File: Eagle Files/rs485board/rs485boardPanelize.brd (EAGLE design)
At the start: 63.5 x 76.7 mm, 100 parts, among them IC1 XC6206P332MR, IC2 MP2562, J1 AVR_SPI_PROG_3X2PTH, J2 RA 6Pin SMD, Q1 CJ3404, Q2 CJ3404, Q3 CJ3404, U1 ATMEGA328P_TQFP, U2 LIS3DH, U3 SP485, X1 RJ45-8P8C-8L-B, X3 RJ45-8P8C-8L-B, Y1 16MHz

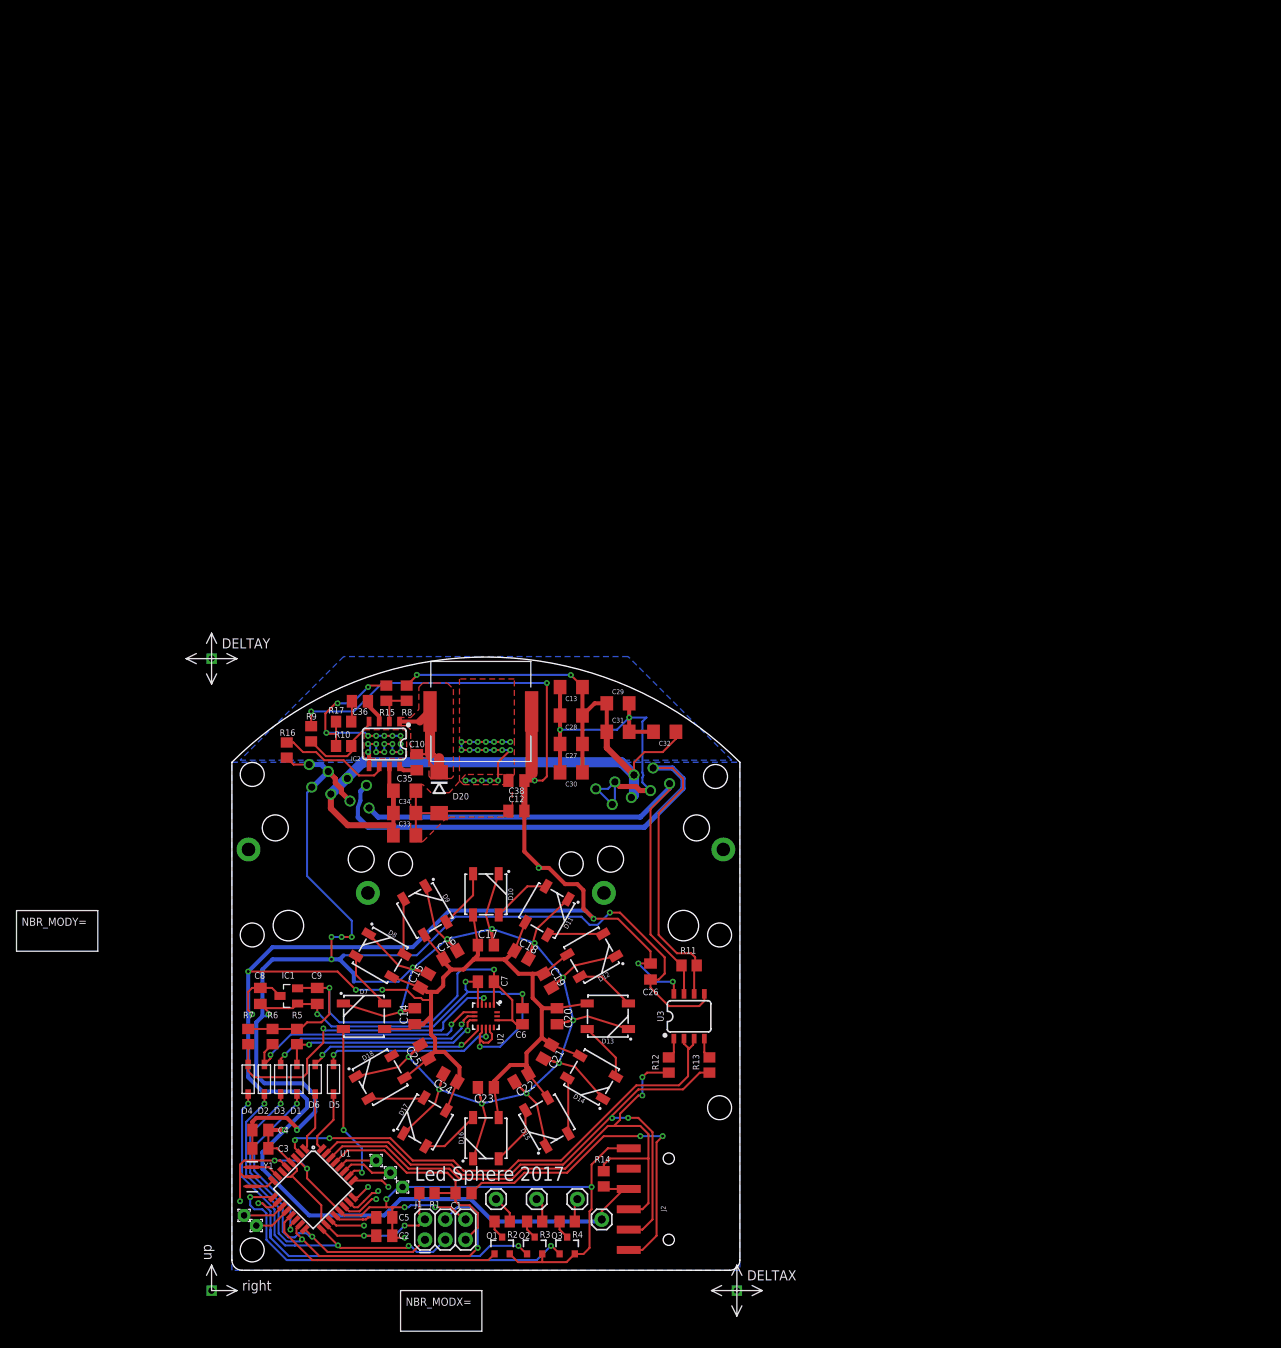
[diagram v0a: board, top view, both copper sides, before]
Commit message: clean up 2*2
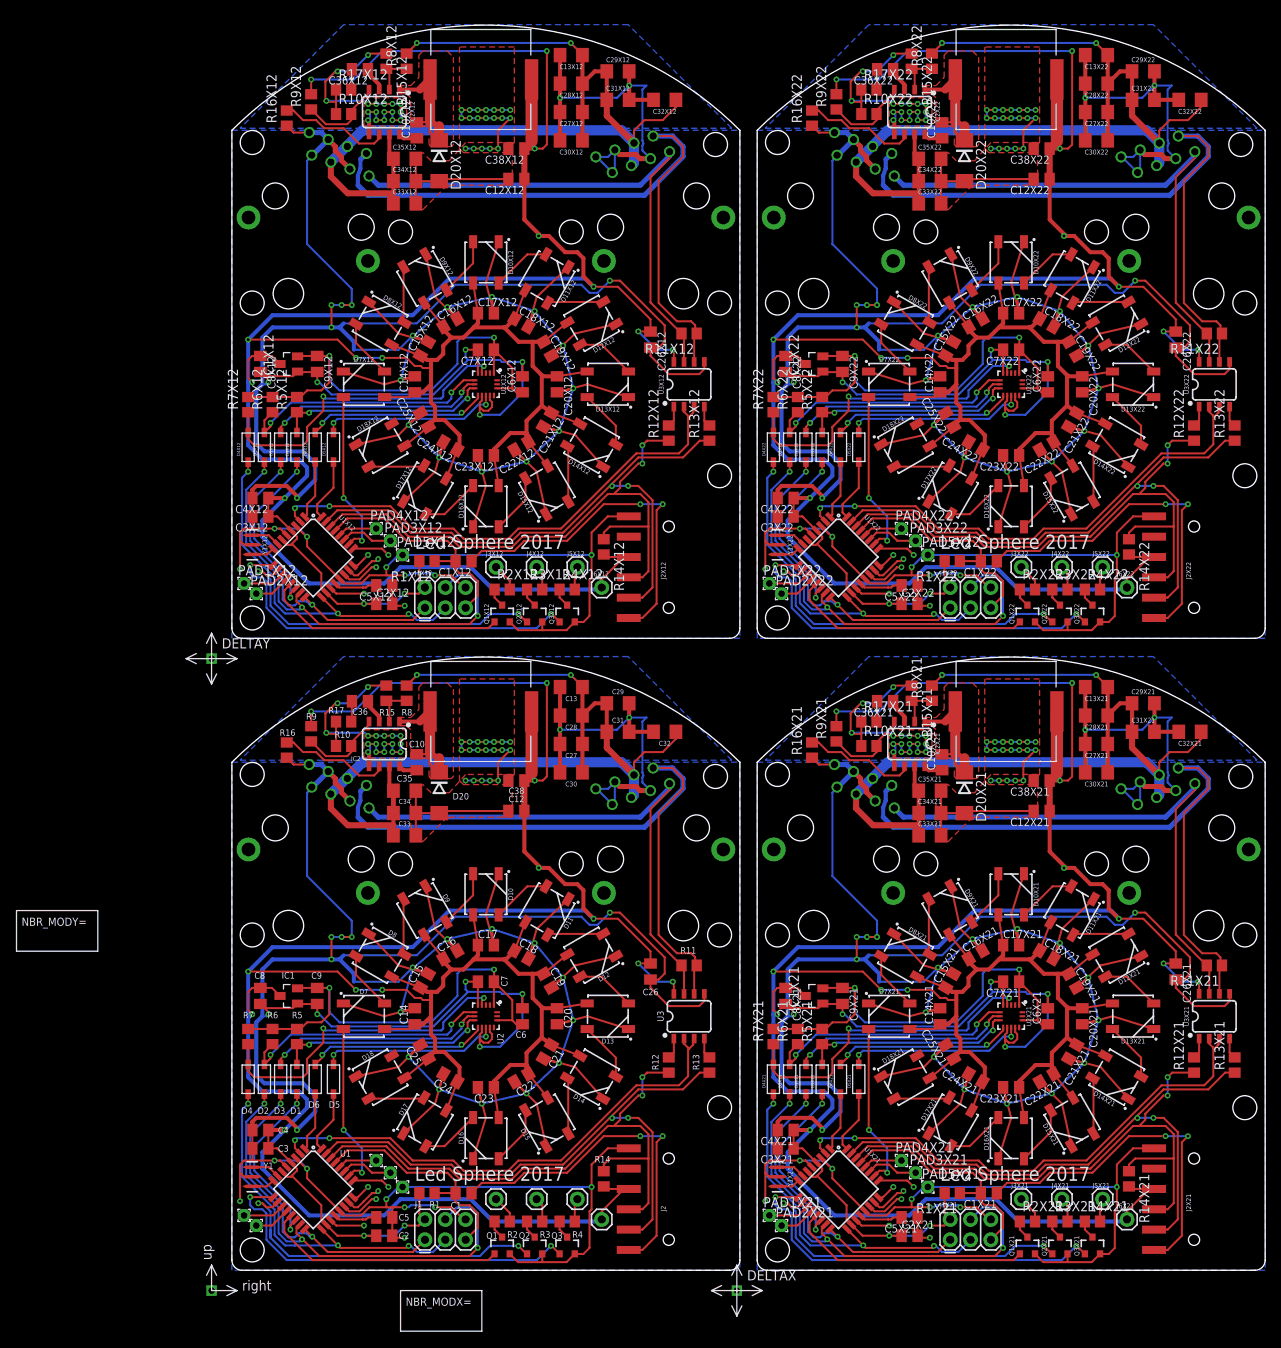
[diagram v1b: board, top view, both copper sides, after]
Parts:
- added C10X12, C10X21, C10X22, C14X12, C14X21, C14X22, C15X12, C15X21, C15X22, C16X12, C16X21, C16X22, C17X12, C17X21, C17X22, C18X12, C18X21, C18X22, C19X12, C19X21, C19X22, C1X12, C1X21, C1X22, C20X12, C20X21, C20X22, C21X12, C21X21, C21X22, C22X12, C22X21, C22X22, C23X12, C23X21, C23X22, C24X12, C24X21, C24X22, C25X12, C25X21, C25X22, C26X12, C26X21, C26X22, C3X12, C3X21, C3X22, C4X12, C4X21, C4X22, C5X12, C5X21, C5X22, C7X12, C7X21, C7X22, C8X12, C8X21, C8X22, C9X12, C9X21, C9X22: 0.1uF, resistor:C0805K
- added C12X12, C12X21, C12X22, C2X12, C2X21, C2X22, C38X12, C38X21, C38X22, C6X12, C6X21, C6X22: 10uF, resistor:C0805K
- added C13X12, C13X21, C13X22, C27X12, C27X21, C27X22, C28X12, C28X21, C28X22, C29X12, C29X21, C29X22, C30X12, C30X21, C30X22, C31X12, C31X21, C31X22, C32X12, C32X21, C32X22, C33X12, C33X21, C33X22, C34X12, C34X21, C34X22, C35X12, C35X21, C35X22: 1uF 100V, SparkFun-Capacitors:1206
- added C36X12, C36X21, C36X22: 150pF, resistor:C0805K
- added D10X12, D10X21, D10X22, D11X12, D11X21, D11X22, D12X12, D12X21, D12X22, D13X12, D13X21, D13X22, D14X12, D14X21, D14X22, D15X12, D15X21, D15X22, D16X12, D16X21, D16X22, D17X12, D17X21, D17X22, D18X12, D18X21, D18X22, D7X12, D7X21, D7X22, D8X12, D8X21, D8X22, D9X12, D9X21, D9X22: WS2812B, SparkFun-LED:WS2812B
- added D1X12, D1X21, D1X22, D2X12, D2X21, D2X22, D3X12, D3X21, D3X22, D4X12, D4X21, D4X22, D5X12, D5X21, D5X22, D6X12, D6X21, D6X22: 5819, adafruit:SOD-123
- added D20X12, D20X21, D20X22: B280-13-F, diode:DO214AA
- added IC1X12, IC1X21, IC1X22: XC6206P332MR, linear:SOT23
- added IC2X12, IC2X21, IC2X22: MP2562, misc:SO08
- added J1X12, J1X21, J1X22: AVR_SPI_PROG_3X2PTH, SparkFun-Connectors:2X3
- added J2X12, J2X21, J2X22: RA 6Pin SMD, SparkFun-Connectors:1X06-SMD_RA_MALE
- added J3X12, J3X21, J3X22, J4X12, J4X21, J4X22, J5X12, J5X21, J5X22, J6X12, J6X21, J6X22: (no value), SparkFun-Connectors:1X01
- added L1X12, L1X21, L1X22: 15uH, misc:SLF12575
- added PAD1X12, PAD1X21, PAD1X22, PAD2X12, PAD2X21, PAD2X22, PAD3X12, PAD3X21, PAD3X22, PAD4X12, PAD4X21, PAD4X22, PAD5X12, PAD5X21, PAD5X22: (no value), wirepad:1,6/0,8
- added Q1X12, Q1X21, Q1X22, Q2X12, Q2X21, Q2X22, Q3X12, Q3X21, Q3X22: CJ3404, SparkFun-DiscreteSemi:SOT23-3
- added R10X12, R10X21, R10X22: 40.2k, resistor:R0805
- added R11X12, R11X21, R11X22: 120, resistor:R0805
- added R12X12, R12X21, R12X22, R13X12, R13X21, R13X22: 1K, resistor:R0805
- added R14X12, R14X21, R14X22, R1X12, R1X21, R1X22, R5X12, R5X21, R5X22, R6X12, R6X21, R6X22, R7X12, R7X21, R7X22: 10K, resistor:R0805
- added R15X12, R15X21, R15X22: 17.4K, resistor:R0805
- added R16X12, R16X21, R16X22: 200K, resistor:R0805
- added R17X12, R17X21, R17X22: 158K, resistor:R0805
- added R2X12, R2X21, R2X22, R3X12, R3X21, R3X22, R4X12, R4X21, R4X22: DNP, resistor:R0805
- added R8X12, R8X21, R8X22: 100K, resistor:R0805
- added R9X12, R9X21, R9X22: 210K, resistor:R0805
- added U1X12, U1X21, U1X22: ATMEGA328P_TQFP, SparkFun-IC-Microcontroller:TQFP32-08
- added U2X12, U2X21, U2X22: LIS3DH, SparkFun-Sensors:LGA-16-3X3
- added U3X12, U3X21, U3X22: SP485, SparkFun-IC-Comms:SO08
- added X1X12, X1X21, X1X22, X3X12, X3X21, X3X22: RJ45-8P8C-8L-B, myownParts:RJ45-SHIELD-DS1128-S80BP
- added Y1X12, Y1X21, Y1X22: 16MHz, SparkFun-Clocks:RESONATOR-SMD-3.2X1.3
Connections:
- new net +24VX12: C13X12.1, C27X12.1, C28X12.1, C29X12.1, C30X12.1, C31X12.1, C32X12.1, C33X12.1, C34X12.1, C35X12.1, IC2X12.7, R8X12.2, X1X12.4, X1X12.5, X3X12.4, X3X12.5
- new net +24VX21: C13X21.1, C27X21.1, C28X21.1, C29X21.1, C30X21.1, C31X21.1, C32X21.1, C33X21.1, C34X21.1, C35X21.1, IC2X21.7, R8X21.2, X1X21.4, X1X21.5, X3X21.4, X3X21.5
- new net +24VX22: C13X22.1, C27X22.1, C28X22.1, C29X22.1, C30X22.1, C31X22.1, C32X22.1, C33X22.1, C34X22.1, C35X22.1, IC2X22.7, R8X22.2, X1X22.4, X1X22.5, X3X22.4, X3X22.5
- new net +3V3X12: C6X12.1, C7X12.1, C9X12.1, IC1X12.2, R5X12.2, R6X12.2, R7X12.2, U2X12.1, U2X12.14
- new net +3V3X21: C6X21.1, C7X21.1, C9X21.1, IC1X21.2, R5X21.2, R6X21.2, R7X21.2, U2X21.1, U2X21.14
- new net +3V3X22: C6X22.1, C7X22.1, C9X22.1, IC1X22.2, R5X22.2, R6X22.2, R7X22.2, U2X22.1, U2X22.14
- new net +5VX12: C12X12.1, C14X12.1, C15X12.1, C16X12.1, C17X12.1, C18X12.1, C19X12.1, C20X12.1, C21X12.1, C22X12.1, C23X12.1, C24X12.1, C25X12.1, C26X12.1, C2X12.1, C38X12.1, C3X12.1, C4X12.1, C8X12.1, D10X12.1, D11X12.1, D12X12.1, D13X12.1, D14X12.1, D15X12.1, D16X12.1, D17X12.1, D18X12.1, D7X12.1, D8X12.1, D9X12.1, IC1X12.3, J1X12.2, J2X12.4, J6X12.1, L1X12.P$2, R14X12.2, R1X12.2, R9X12.2, U1X12.18, U1X12.4, U1X12.6, U3X12.8
- new net +5VX21: C12X21.1, C14X21.1, C15X21.1, C16X21.1, C17X21.1, C18X21.1, C19X21.1, C20X21.1, C21X21.1, C22X21.1, C23X21.1, C24X21.1, C25X21.1, C26X21.1, C2X21.1, C38X21.1, C3X21.1, C4X21.1, C8X21.1, D10X21.1, D11X21.1, D12X21.1, D13X21.1, D14X21.1, D15X21.1, D16X21.1, D17X21.1, D18X21.1, D7X21.1, D8X21.1, D9X21.1, IC1X21.3, J1X21.2, J2X21.4, J6X21.1, L1X21.P$2, R14X21.2, R1X21.2, R9X21.2, U1X21.18, U1X21.4, U1X21.6, U3X21.8
- new net +5VX22: C12X22.1, C14X22.1, C15X22.1, C16X22.1, C17X22.1, C18X22.1, C19X22.1, C20X22.1, C21X22.1, C22X22.1, C23X22.1, C24X22.1, C25X22.1, C26X22.1, C2X22.1, C38X22.1, C3X22.1, C4X22.1, C8X22.1, D10X22.1, D11X22.1, D12X22.1, D13X22.1, D14X22.1, D15X22.1, D16X22.1, D17X22.1, D18X22.1, D7X22.1, D8X22.1, D9X22.1, IC1X22.3, J1X22.2, J2X22.4, J6X22.1, L1X22.P$2, R14X22.2, R1X22.2, R9X22.2, U1X22.18, U1X22.4, U1X22.6, U3X22.8
- new net A3X12: D7X12.4, U1X12.26
- new net A3X21: D7X21.4, U1X21.26
- new net A3X22: D7X22.4, U1X22.26
- new net A4X12: PAD3X12.1, U1X12.27
- new net A4X21: PAD3X21.1, U1X21.27
- new net A4X22: PAD3X22.1, U1X22.27
- new net A5X12: PAD4X12.1, U1X12.28
- new net A5X21: PAD4X21.1, U1X21.28
- new net A5X22: PAD4X22.1, U1X22.28
- new net AREFX12: C5X12.2, U1X12.20
- new net AREFX21: C5X21.2, U1X21.20
- new net AREFX22: C5X22.2, U1X22.20
- new net BSTX12: C10X12.1, IC2X12.8
- new net BSTX21: C10X21.1, IC2X21.8
- new net BSTX22: C10X22.1, IC2X22.8
- new net COMPX12: C36X12.1, IC2X12.3
- new net COMPX21: C36X21.1, IC2X21.3
- new net COMPX22: C36X22.1, IC2X22.3
- new net D2X12: D5X12.C, U1X12.32
- new net D2X21: D5X21.C, U1X21.32
- new net D2X22: D5X22.C, U1X22.32
- new net D3X12: D6X12.C, U1X12.1
- new net D3X21: D6X21.C, U1X21.1
- new net D3X22: D6X22.C, U1X22.1
- new net D5X12: Q3X12.1, U1X12.9
- new net D5X21: Q3X21.1, U1X21.9
- new net D5X22: Q3X22.1, U1X22.9
- new net D6X12: Q2X12.1, U1X12.10
- new net D6X21: Q2X21.1, U1X21.10
- new net D6X22: Q2X22.1, U1X22.10
- new net D7X12: PAD1X12.1, U1X12.11
- new net D7X21: PAD1X21.1, U1X21.11
- new net D7X22: PAD1X22.1, U1X22.11
- new net D8X12: PAD2X12.1, U1X12.12
- new net D8X21: PAD2X21.1, U1X21.12
- new net D8X22: PAD2X22.1, U1X22.12
- new net D9X12: Q1X12.1, U1X12.13
- new net D9X21: Q1X21.1, U1X21.13
- new net D9X22: Q1X22.1, U1X22.13
- new net DIRX12: U1X12.2, U3X12.2, U3X12.3
- new net DIRX21: U1X21.2, U3X21.2, U3X21.3
- new net DIRX22: U1X22.2, U3X22.2, U3X22.3
- new net ENX12: IC2X12.2, R15X12.2, R8X12.1
- new net ENX21: IC2X21.2, R15X21.2, R8X21.1
- new net ENX22: IC2X22.2, R15X22.2, R8X22.1
- new net FBX12: IC2X12.4, R10X12.2, R9X12.1
- new net FBX21: IC2X21.4, R10X21.2, R9X21.1
- new net FBX22: IC2X22.4, R10X22.2, R9X22.1
- new net FREQX12: IC2X12.6, R16X12.2
- new net FREQX21: IC2X21.6, R16X21.2
- new net FREQX22: IC2X22.6, R16X22.2
- new net GNDX12: C12X12.2, C13X12.2, C14X12.2, C15X12.2, C16X12.2, C17X12.2, C18X12.2, C19X12.2, C20X12.2, C21X12.2, C22X12.2, C23X12.2, C24X12.2, C25X12.2, C26X12.2, C27X12.2, C28X12.2, C29X12.2, C2X12.2, C30X12.2, C31X12.2, C32X12.2, C33X12.2, C34X12.2, C35X12.2, C38X12.2, C3X12.2, C4X12.2, C5X12.1, C6X12.2, C7X12.2, C8X12.2, C9X12.2, D10X12.3, D11X12.3, D12X12.3, D13X12.3, D14X12.3, D15X12.3, D16X12.3, D17X12.3, D18X12.3, D20X12.A, D7X12.3, D8X12.3, D9X12.3, IC1X12.1, IC2X12.5, J1X12.6, J2X12.6, PAD5X12.1, Q1X12.2, Q2X12.2, Q3X12.2, R10X12.1, R15X12.1, R16X12.1, R17X12.1, U1X12.21, U1X12.3, U1X12.5, U2X12.10, U2X12.12, U2X12.5, U3X12.5, X1X12.3, X1X12.6, X1X12.7, X1X12.8, X3X12.3, X3X12.6, X3X12.7, X3X12.8, Y1X12.2
- new net GNDX21: C12X21.2, C13X21.2, C14X21.2, C15X21.2, C16X21.2, C17X21.2, C18X21.2, C19X21.2, C20X21.2, C21X21.2, C22X21.2, C23X21.2, C24X21.2, C25X21.2, C26X21.2, C27X21.2, C28X21.2, C29X21.2, C2X21.2, C30X21.2, C31X21.2, C32X21.2, C33X21.2, C34X21.2, C35X21.2, C38X21.2, C3X21.2, C4X21.2, C5X21.1, C6X21.2, C7X21.2, C8X21.2, C9X21.2, D10X21.3, D11X21.3, D12X21.3, D13X21.3, D14X21.3, D15X21.3, D16X21.3, D17X21.3, D18X21.3, D20X21.A, D7X21.3, D8X21.3, D9X21.3, IC1X21.1, IC2X21.5, J1X21.6, J2X21.6, PAD5X21.1, Q1X21.2, Q2X21.2, Q3X21.2, R10X21.1, R15X21.1, R16X21.1, R17X21.1, U1X21.21, U1X21.3, U1X21.5, U2X21.10, U2X21.12, U2X21.5, U3X21.5, X1X21.3, X1X21.6, X1X21.7, X1X21.8, X3X21.3, X3X21.6, X3X21.7, X3X21.8, Y1X21.2
- new net GNDX22: C12X22.2, C13X22.2, C14X22.2, C15X22.2, C16X22.2, C17X22.2, C18X22.2, C19X22.2, C20X22.2, C21X22.2, C22X22.2, C23X22.2, C24X22.2, C25X22.2, C26X22.2, C27X22.2, C28X22.2, C29X22.2, C2X22.2, C30X22.2, C31X22.2, C32X22.2, C33X22.2, C34X22.2, C35X22.2, C38X22.2, C3X22.2, C4X22.2, C5X22.1, C6X22.2, C7X22.2, C8X22.2, C9X22.2, D10X22.3, D11X22.3, D12X22.3, D13X22.3, D14X22.3, D15X22.3, D16X22.3, D17X22.3, D18X22.3, D20X22.A, D7X22.3, D8X22.3, D9X22.3, IC1X22.1, IC2X22.5, J1X22.6, J2X22.6, PAD5X22.1, Q1X22.2, Q2X22.2, Q3X22.2, R10X22.1, R15X22.1, R16X22.1, R17X22.1, U1X22.21, U1X22.3, U1X22.5, U2X22.10, U2X22.12, U2X22.5, U3X22.5, X1X22.3, X1X22.6, X1X22.7, X1X22.8, X3X22.3, X3X22.6, X3X22.7, X3X22.8, Y1X22.2
- new net INT1X12: D5X12.A, U2X12.11
- new net INT1X21: D5X21.A, U2X21.11
- new net INT1X22: D5X22.A, U2X22.11
- new net INT2X12: D6X12.A, U2X12.9
- new net INT2X21: D6X21.A, U2X21.9
- new net INT2X22: D6X22.A, U2X22.9
- new net MISOX12: D3X12.C, J1X12.1, U1X12.16
- new net MISOX21: D3X21.C, J1X21.1, U1X21.16
- new net MISOX22: D3X22.C, J1X22.1, U1X22.16
- new net MISO_3.3VX12: D3X12.A, U2X12.7
- new net MISO_3.3VX21: D3X21.A, U2X21.7
- new net MISO_3.3VX22: D3X22.A, U2X22.7
- new net MOSIX12: D2X12.C, J1X12.4, U1X12.15
- new net MOSIX21: D2X21.C, J1X21.4, U1X21.15
- new net MOSIX22: D2X22.C, J1X22.4, U1X22.15
- new net MOSI_3.3VX12: D2X12.A, R6X12.1, U2X12.6
- new net MOSI_3.3VX21: D2X21.A, R6X21.1, U2X21.6
- new net MOSI_3.3VX22: D2X22.A, R6X22.1, U2X22.6
- new net N$10X12: D10X12.2, D11X12.4
- new net N$10X21: D10X21.2, D11X21.4
- new net N$10X22: D10X22.2, D11X22.4
- new net N$11X12: D11X12.2, D12X12.4
- new net N$11X21: D11X21.2, D12X21.4
- new net N$11X22: D11X22.2, D12X22.4
- new net N$12X12: D12X12.2, D13X12.4
- new net N$12X21: D12X21.2, D13X21.4
- new net N$12X22: D12X22.2, D13X22.4
- new net N$13X12: D13X12.2, D14X12.4
- new net N$13X21: D13X21.2, D14X21.4
- new net N$13X22: D13X22.2, D14X22.4
- new net N$14X12: D14X12.2, D15X12.4
- new net N$14X21: D14X21.2, D15X21.4
- new net N$14X22: D14X22.2, D15X22.4
- new net N$15X12: D15X12.2, D16X12.4
- new net N$15X21: D15X21.2, D16X21.4
- new net N$15X22: D15X22.2, D16X22.4
- new net N$16X12: D16X12.2, D17X12.4
- new net N$16X21: D16X21.2, D17X21.4
- new net N$16X22: D16X22.2, D17X22.4
- new net N$17X12: D17X12.2, D18X12.4
- new net N$17X21: D17X21.2, D18X21.4
- new net N$17X22: D17X22.2, D18X22.4
- new net N$1X12: Q1X12.3, R2X12.1
- new net N$1X21: Q1X21.3, R2X21.1
- new net N$1X22: Q1X22.3, R2X22.1
- new net N$25X12: C36X12.2, R17X12.2
- new net N$25X21: C36X21.2, R17X21.2
- new net N$25X22: C36X22.2, R17X22.2
- new net N$2X12: D7X12.2, D8X12.4
- new net N$2X21: D7X21.2, D8X21.4
- new net N$2X22: D7X22.2, D8X22.4
- new net N$30X12: R12X12.2, U3X12.1
- new net N$30X21: R12X21.2, U3X21.1
- new net N$30X22: R12X22.2, U3X22.1
- new net N$31X12: R13X12.2, U3X12.4
- new net N$31X21: R13X21.2, U3X21.4
- new net N$31X22: R13X22.2, U3X22.4
- new net N$3X12: D8X12.2, D9X12.4
- new net N$3X21: D8X21.2, D9X21.4
- new net N$3X22: D8X22.2, D9X22.4
- new net N$4X12: J3X12.1, R2X12.2
- new net N$4X21: J3X21.1, R2X21.2
- new net N$4X22: J3X22.1, R2X22.2
- new net N$5X12: Q2X12.3, R3X12.1
- new net N$5X21: Q2X21.3, R3X21.1
- new net N$5X22: Q2X22.3, R3X22.1
- new net N$6X12: J4X12.1, R3X12.2
- new net N$6X21: J4X21.1, R3X21.2
- new net N$6X22: J4X22.1, R3X22.2
- new net N$7X12: Q3X12.3, R4X12.1
- new net N$7X21: Q3X21.3, R4X21.1
- new net N$7X22: Q3X22.3, R4X22.1
- new net N$8X12: J5X12.1, R4X12.2
- new net N$8X21: J5X21.1, R4X21.2
- new net N$8X22: J5X22.1, R4X22.2
- new net N$9X12: D10X12.4, D9X12.2
- new net N$9X21: D10X21.4, D9X21.2
- new net N$9X22: D10X22.4, D9X22.2
- new net RESETX12: C1X12.2, J1X12.5, R1X12.1, U1X12.29
- new net RESETX21: C1X21.2, J1X21.5, R1X21.1, U1X21.29
- new net RESETX22: C1X22.2, J1X22.5, R1X22.1, U1X22.29
- new net RESET_EXTX12: C1X12.1, J2X12.1
- new net RESET_EXTX21: C1X21.1, J2X21.1
- new net RESET_EXTX22: C1X22.1, J2X22.1
- new net RS485AX12: R11X12.1, U3X12.6, X1X12.2, X3X12.2
- new net RS485AX21: R11X21.1, U3X21.6, X1X21.2, X3X21.2
- new net RS485AX22: R11X22.1, U3X22.6, X1X22.2, X3X22.2
- new net RS485BX12: R11X12.2, U3X12.7, X1X12.1, X3X12.1
- new net RS485BX21: R11X21.2, U3X21.7, X1X21.1, X3X21.1
- new net RS485BX22: R11X22.2, U3X22.7, X1X22.1, X3X22.1
- new net RXX12: J2X12.3, R12X12.1, R14X12.1, U1X12.30
- new net RXX21: J2X21.3, R12X21.1, R14X21.1, U1X21.30
- new net RXX22: J2X22.3, R12X22.1, R14X22.1, U1X22.30
- new net SCKX12: D4X12.C, J1X12.3, U1X12.17
- new net SCKX21: D4X21.C, J1X21.3, U1X21.17
- new net SCKX22: D4X22.C, J1X22.3, U1X22.17
- new net SCK_3.3VX12: D4X12.A, R7X12.1, U2X12.4
- new net SCK_3.3VX21: D4X21.A, R7X21.1, U2X21.4
- new net SCK_3.3VX22: D4X22.A, R7X22.1, U2X22.4
- new net SSX12: D1X12.C, U1X12.14
- new net SSX21: D1X21.C, U1X21.14
- new net SSX22: D1X22.C, U1X22.14
- new net SS_3.3VX12: D1X12.A, R5X12.1, U2X12.8
- new net SS_3.3VX21: D1X21.A, R5X21.1, U2X21.8
- new net SS_3.3VX22: D1X22.A, R5X22.1, U2X22.8
- new net SWX12: C10X12.2, D20X12.C, IC2X12.1, L1X12.P$1
- new net SWX21: C10X21.2, D20X21.C, IC2X21.1, L1X21.P$1
- new net SWX22: C10X22.2, D20X22.C, IC2X22.1, L1X22.P$1
- new net TXX12: J2X12.2, R13X12.1, U1X12.31
- new net TXX21: J2X21.2, R13X21.1, U1X21.31
- new net TXX22: J2X22.2, R13X22.1, U1X22.31
- new net XTAL1X12: U1X12.7, Y1X12.1
- new net XTAL1X21: U1X21.7, Y1X21.1
- new net XTAL1X22: U1X22.7, Y1X22.1
- new net XTAL2X12: U1X12.8, Y1X12.3
- new net XTAL2X21: U1X21.8, Y1X21.3
- new net XTAL2X22: U1X22.8, Y1X22.3
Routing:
- net GNDX22: track 0.00 -> 654.9 mm, vias 0 -> 70
- net GNDX21: track 0.00 -> 654.9 mm, vias 0 -> 70
- net GNDX12: track 0.00 -> 654.9 mm, vias 0 -> 70
- net +5VX21: track 0.00 -> 417.0 mm, vias 0 -> 14
- net +5VX22: track 0.00 -> 417.0 mm, vias 0 -> 14
- net +5VX12: track 0.00 -> 417.0 mm, vias 0 -> 14
- net +24VX22: track 0.00 -> 119.4 mm, vias 0 -> 2
- net +24VX12: track 0.00 -> 119.4 mm, vias 0 -> 2
- net +24VX21: track 0.00 -> 119.4 mm, vias 0 -> 2
- net RS485AX21: track 0.00 -> 88.7 mm
- net RS485AX22: track 0.00 -> 88.7 mm
- net RS485AX12: track 0.00 -> 88.7 mm
- net TXX22: track 0.00 -> 75.9 mm, vias 0 -> 2
- net TXX21: track 0.00 -> 75.9 mm, vias 0 -> 2
- net TXX12: track 0.00 -> 75.9 mm, vias 0 -> 2
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- added copper zone on layer 1, net GNDX12
- added copper zone on layer 16, net GNDX12
- added copper zone on layer 1, net GNDX21
- added copper zone on layer 16, net GNDX21
- added copper zone on layer 1, net GNDX22
- added copper zone on layer 16, net GNDX22
- added copper zone on layer 1, net SWX12
- added copper zone on layer 1, net SWX21
- added copper zone on layer 1, net SWX22
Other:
- board size 63.5 x 76.7 mm -> 129.2 x 155.6 mm
- board text added: "C14"
- board text added: "C15"
- board text added: "C16"
- board text added: "C17"
- board text added: "C18"
- board text added: "C19"
- board text added: "C20"
- board text added: "C21"
- board text added: "C22"
- board text added: "C23"
- board text added: "C24"
- board text added: "C25"
- board text added: "C32"
- board text added: "D10"
- board text added: "D11"
- board text added: "D12"
- board text added: "D13"
- board text added: "D14"
- board text added: "D15"
- board text added: "D16"
- board text added: "D17"
- board text added: "D18"
- board text added: "D7"
- board text added: "D8"
- board text added: "D9"
- board text added: "J2"
- board text added: "Think Create LLC'"
